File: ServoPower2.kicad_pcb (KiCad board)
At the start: 2 copper layers, 26 x 57.2 mm, 16 parts, among them J1 Conn_01x03, J10 Conn_01x03, J11 Conn_01x03, J12 Conn_01x03, J13 Conn_01x02, J14 Conn_01x02, J15 Conn_01x02, J2 Conn_01x03, J3 Conn_01x03, J4 Conn_01x03, J5 Conn_01x03, J6 Conn_01x03, J7 Conn_01x03, J8 Conn_01x03, J9 Conn_01x03

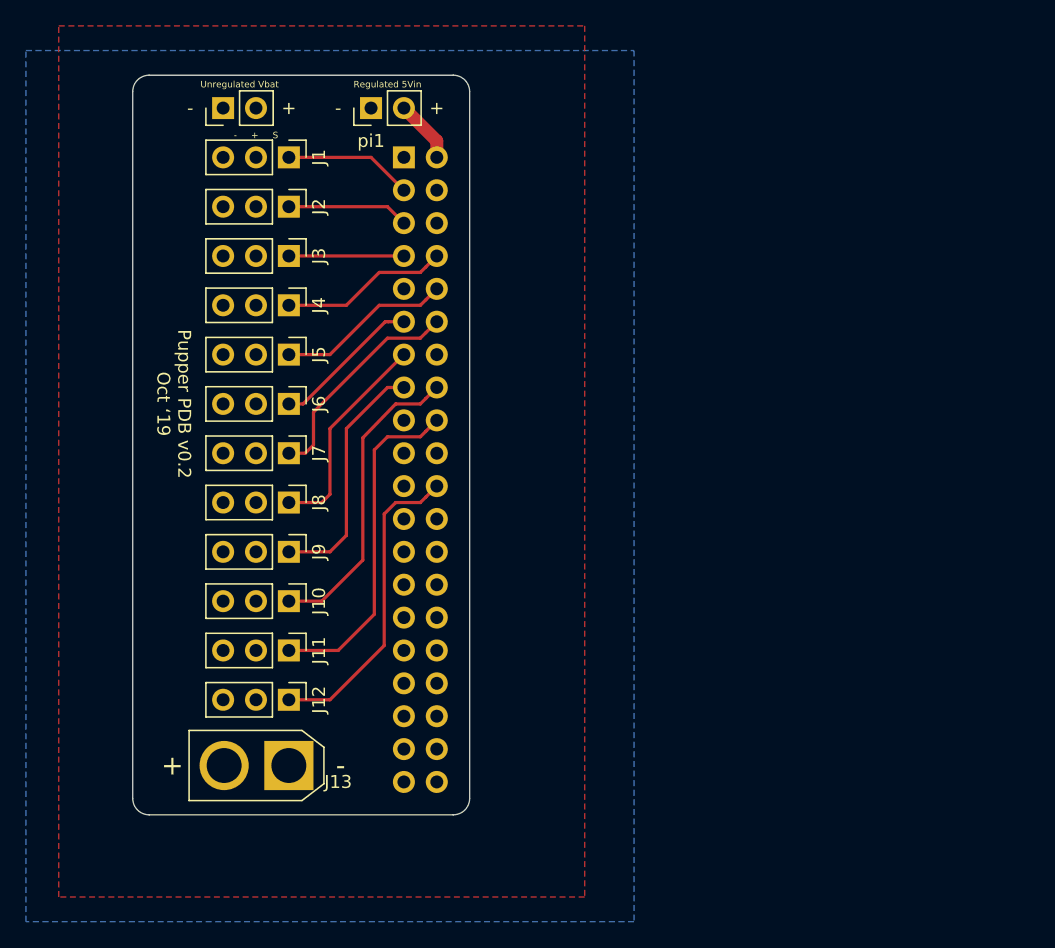
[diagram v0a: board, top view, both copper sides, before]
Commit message: pdb
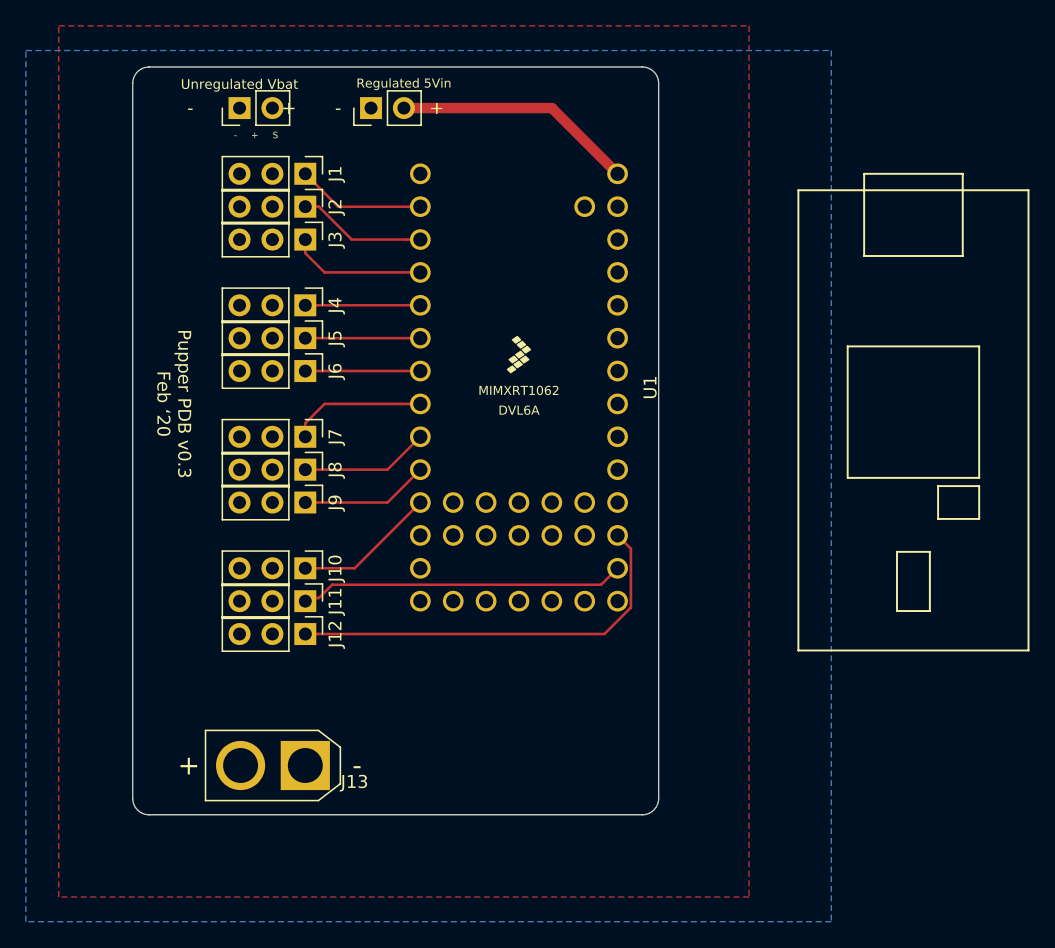
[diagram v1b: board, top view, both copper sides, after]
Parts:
- removed pi1: pi, Connector_PinSocket_2.54mm:PinSocket_2x20_P2.54mm_Vertical
- added U1: Teensy4.0, teensy:Teensy40, F.Cu at (143.5, 82.5)
- moved J12 5.24 mm to (157.5, 104.1)
- moved J11 4.02 mm to (157.5, 101.6)
- moved J9 4.02 mm to (157.5, 94.0)
- moved J6 2.84 mm to (157.5, 83.8)
- moved J8 2.84 mm to (157.5, 91.4)
- moved J10 2.84 mm to (157.5, 99.1)
- moved J3 1.80 mm to (157.5, 73.7)
- moved J1 1.80 mm to (157.5, 68.6)
- moved J5 1.80 mm to (157.5, 81.3)
- moved J7 1.80 mm to (157.5, 88.9)
- moved J14 1.27 mm to (152.4, 63.5)
- moved J13 1.27 mm to (157.5, 114.3)
- moved J2 1.27 mm to (157.5, 71.1)
- moved J4 1.27 mm to (157.5, 78.7)
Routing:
- net +5V: track 4.86 -> 18.6 mm
- net /S41: track 23.8 -> 11.0 mm
- net /S33: track 19.0 -> 9.94 mm
- net /S43: track 24.2 -> 32.0 mm
- net /S32: track 16.6 -> 9.94 mm
- net /S31: track 17.1 -> 10.6 mm
- net /S22: track 13.5 -> 8.89 mm
- net /S21: track 13.0 -> 8.89 mm
- net /S23: track 11.5 -> 8.89 mm
- net /S13: track 8.89 -> 10.6 mm
- net /S42: track 26.2 -> 25.2 mm
- net /S12: track 9.42 -> 9.94 mm
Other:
- board size 26 x 57.2 mm -> 40.6 x 57.8 mm
- net class Power: trace_width 1 -> 0.8
- board text added: "Pupper PDB v0.3 Feb ‘20"
- board text removed: "Pupper PDB v0.2 Oct ‘19"
